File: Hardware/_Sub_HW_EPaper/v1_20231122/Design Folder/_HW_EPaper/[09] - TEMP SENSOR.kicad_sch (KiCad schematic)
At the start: 3 parts, among them U901 MCP9700T-E/TT

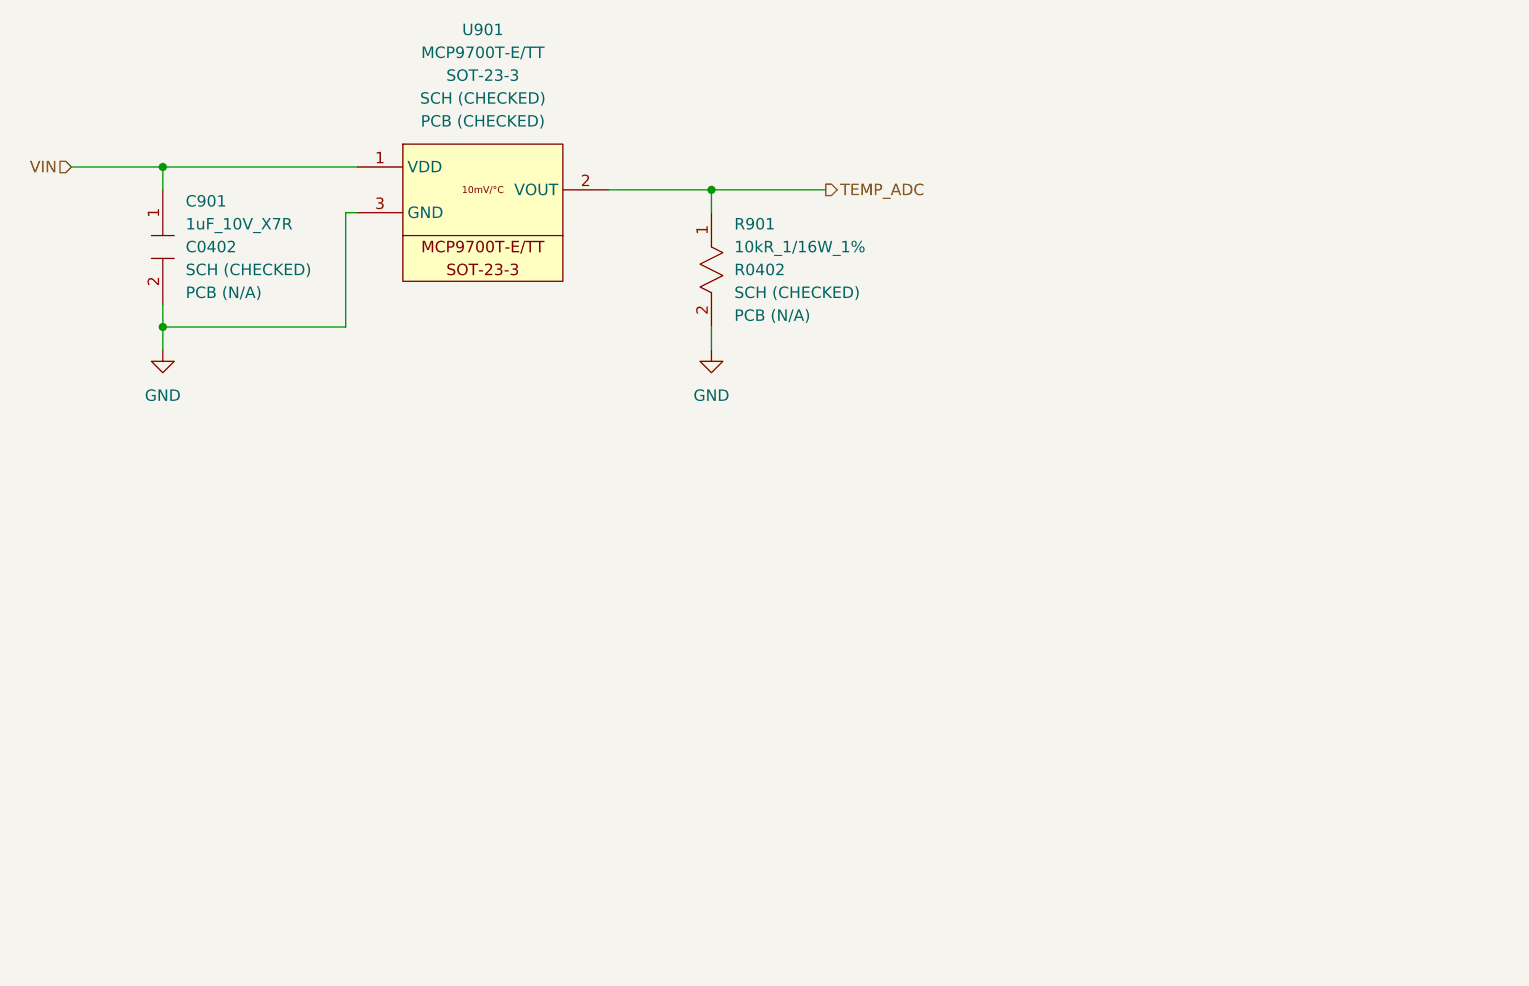
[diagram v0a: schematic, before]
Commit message: Updating file templates and structures...
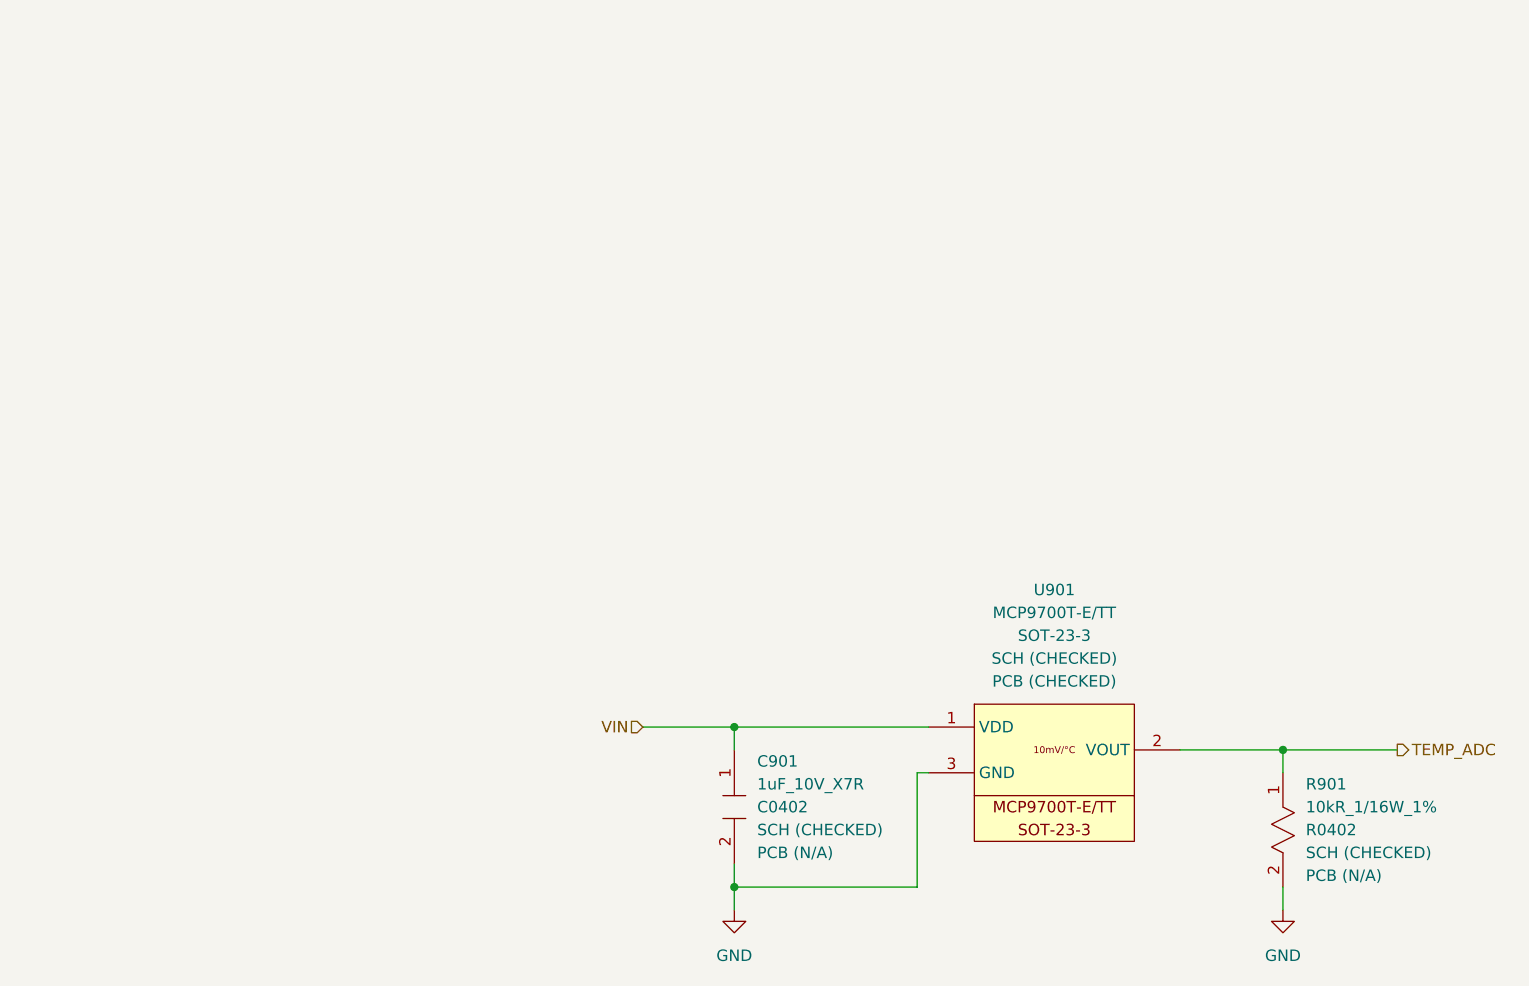
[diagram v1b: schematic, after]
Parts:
- C901: Manufacturer (none) -> Murata Electronics; Part Number GRM155Z71A105KE01D -> (none); Part Number (Manufacturer) (none) -> GRM155Z71A105KE01D; Part Number (Vendor) (none) -> 490-GRM155Z71A105KE01DTR-ND; Vendor (none) -> Digikey
- R901: Manufacturer (none) -> Bourns Inc.; Part Number CR0402-FX-1002GLF -> (none); Part Number (Manufacturer) (none) -> CR0402-FX-1002GLF; Part Number (Vendor) (none) -> CR0402-FX-1002GLFTR-ND; Vendor (none) -> Digikey
- U901: Manufacturer (none) -> Microchip Technology; Part Number MCP9700T-E/TT -> (none); Part Number (Manufacturer) (none) -> MCP9700T-E/TT; Part Number (Vendor) (none) -> MCP9700T-E/TTTR-ND; Vendor (none) -> Digikey
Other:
- moved on the sheet: C901, R901, U901
